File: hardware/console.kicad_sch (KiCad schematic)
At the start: 35 parts, among them J1 USB-C_Module, J2 4.5V_BAT, J3 SWD, J4 UART, Q1 AO3401A, SW1 SW_LEFT, SW2 SW_RIGHT, SW3 SW_UP, SW4 SW_DOWN, SW5 SW_A, SW6 SW_B, U1 STM32G030C8T6, U2 XC6206P332MR

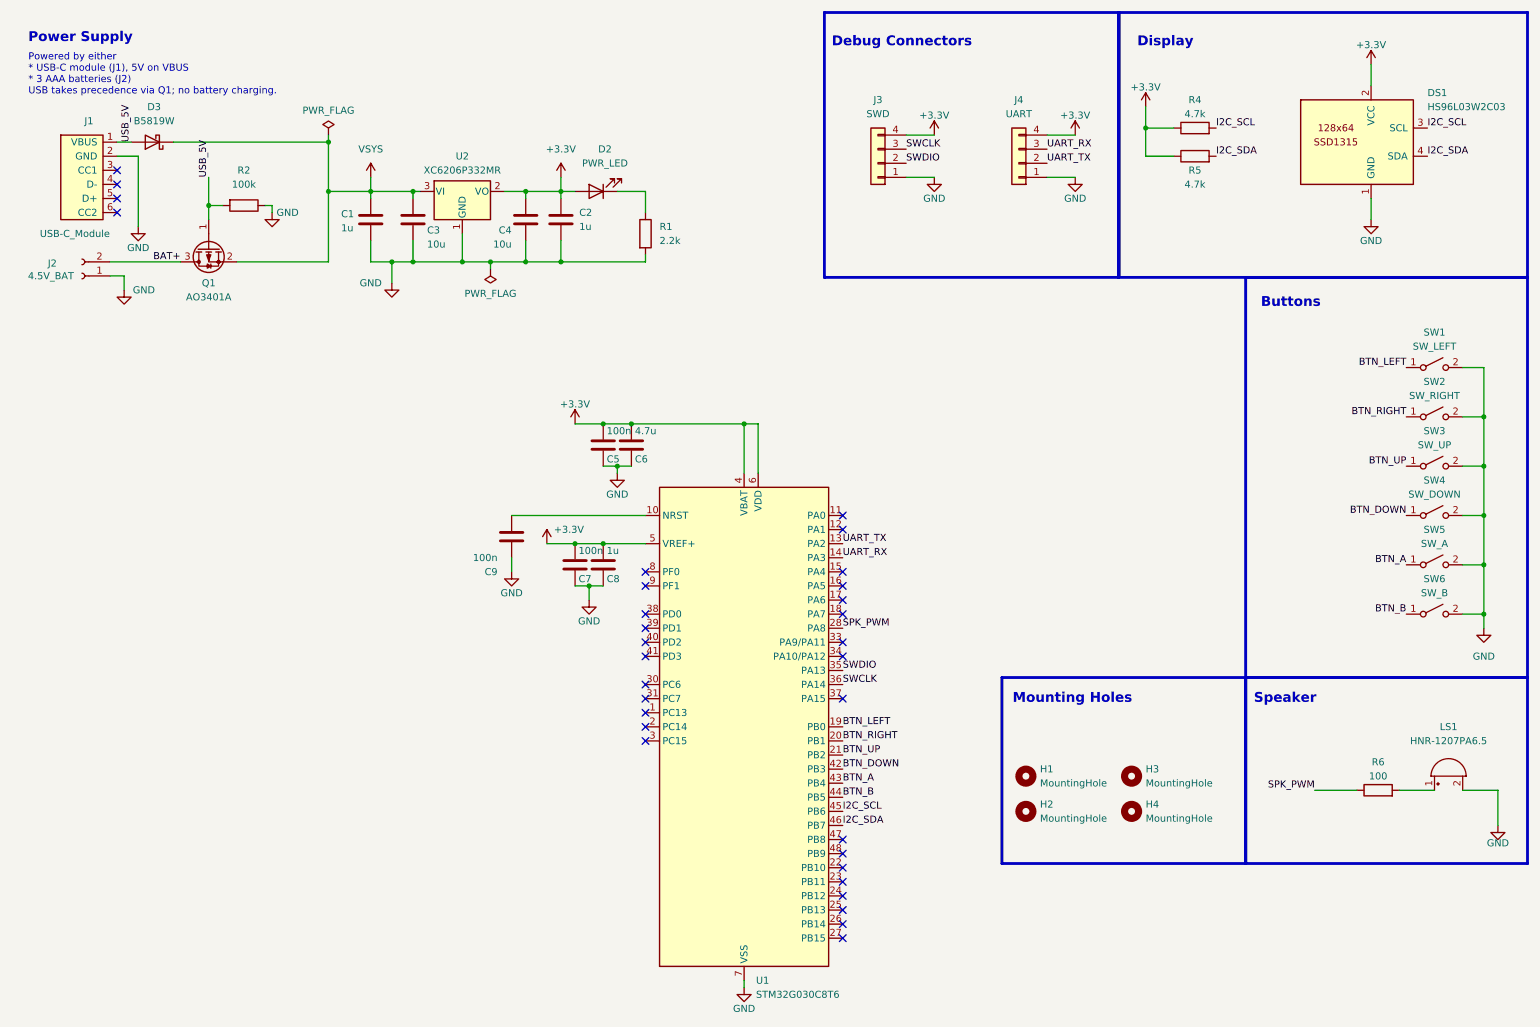
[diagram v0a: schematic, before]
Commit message: checkpoint
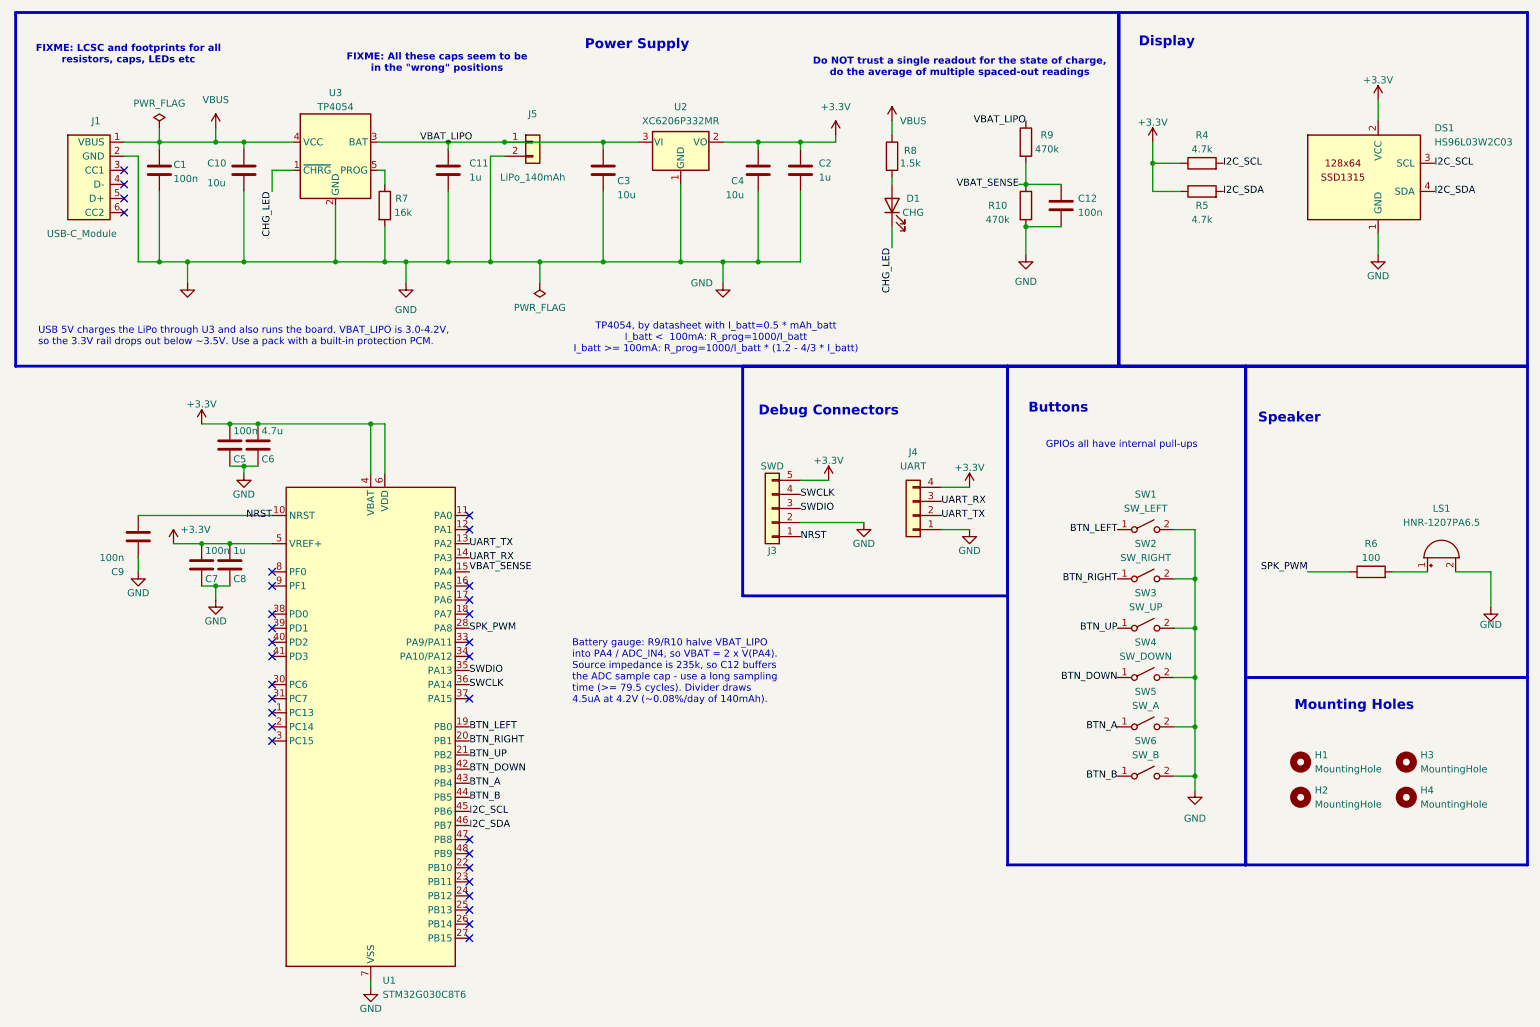
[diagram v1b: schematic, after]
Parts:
- removed D2: PWR_LED, LED_SMD:LED_0603_1608Metric, symbol Device:LED
- removed D3: B5819W, Diode_SMD:D_SOD-123, symbol Device:D_Schottky
- removed J2: 4.5V_BAT, Connector_JST:JST_PH_S2B-PH-K_1x02_P2.00mm_Horizontal, symbol Connector:Conn_01x02_Socket
- removed J3: SWD, Connector_PinHeader_2.54mm:PinHeader_1x04_P2.54mm_Vertical, symbol Connector_Generic:Conn_01x04
- removed Q1: AO3401A, Package_TO_SOT_SMD:SOT-23, symbol Transistor_FET:Q_PMOS_GSD
- removed R1: 2.2k, Resistor_SMD:R_0402_1005Metric, symbol Device:R
- removed R2: 100k, Resistor_SMD:R_0402_1005Metric, symbol Device:R
- added C10: 10u, Capacitor_SMD:C_0805_2012Metric, symbol Device:C
- added C11: 1u, Capacitor_SMD:C_0402_1005Metric, symbol Device:C
- added C12: 100n, Capacitor_SMD:C_0402_1005Metric, symbol Device:C
- added D1: CHG, LED_SMD:LED_0603_1608Metric, symbol Device:LED
- added J3: SWD, Connector_PinHeader_2.54mm:PinHeader_1x05_P2.54mm_Vertical, symbol Connector_Generic:Conn_01x05
- added J5: LiPo_140mAh, Connector_JST:JST_PH_B2B-PH-K_1x02_P2.00mm_Vertical, symbol Connector_Generic:Conn_01x02
- added R10, R9: 470k, Resistor_SMD:R_0402_1005Metric, symbol Device:R
- added R7: 16k, Resistor_SMD:R_0402_1005Metric, symbol Device:R
- added R8: 1.5k, Resistor_SMD:R_0402_1005Metric, symbol Device:R
- added U3: TP4054, Package_TO_SOT_SMD:SOT-23-5, symbol console:TP4054
- C1: value 1u -> 100n
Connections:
- net +3.3V: now also J3.5 (Pin_5)
- net GND: now also C10.2, C11.2, C12.2, J3.2 (Pin_2), J5.2 (Pin_2), R10.2, R7.2, U3.2 (GND)
- net SWCLK: now also J3.4 (Pin_4)
- net SWDIO: now also J3.3 (Pin_3)
- net NRST: now reaches C9.1, U1.10 (NRST)
- net NRST: now also J3.1 (Pin_1)
- net VBAT_SENSE: now reaches U1.15 (PA4)
- net VBAT_SENSE: now also C12.1, R10.1, R9.2
- net USB_5V renamed VBUS
- net VBUS: now also C1.1, C10.1, R8.1, U3.4 (VCC)
- net VSYS renamed VBAT_LIPO
- net VBAT_LIPO: now also C11.1, J5.1 (Pin_1), R9.1, U3.3 (BAT); no longer C1.1
- new net: R7.1, U3.5 (PROG)
- new net: D1.2 (A), R8.2
- new net CHG_LED: D1.1 (K), U3.1 (~{CHRG})
- no-connect marks 32 -> 31
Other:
- note added: "Battery gauge: R9/R10 halve VBAT_LIPO into PA4 / ADC_IN4, so VBAT = 2 x V(PA4). Source impedance is 235k, so C12 buffers the ADC sample cap - use a long sampling time (>= 79.5 cycles). Divider draws 4.5uA at 4.2V (~0.08%/day of 140mAh)."
- note added: "Do NOT trust a single readout for the state of charge, do the average of multiple spaced-out readings"
- note added: "FIXME: All these caps seem to be in the "wrong" positions"
- note added: "FIXME: LCSC and footprints for all resistors, caps, LEDs etc"
- note added: "GPIOs all have internal pull-ups"
- note added: "TP4054, by datasheet with I_batt=0.5 * mAh_batt I_batt < 100mA: R_prog=1000/I_batt I_batt >= 100mA: R_prog=1000/I_batt * (1.2 - 4/3 * I_batt)"
- note added: "USB 5V charges the LiPo through U3 and also runs the board. VBAT_LIPO is 3.0-4.2V, so the 3.3V rail drops out below ~3.5V. Use a pack with a built-in protection PCM."
- note removed: "Powered by either * USB-C module (J1), 5V on VBUS * 3 AAA batteries (J2) USB takes precedence via Q1; no battery charging."
- title: (none) -> MicroConsole
- moved on the sheet: C1, C2, C3, C4, C5, C6, C7, C8, C9, DS1, H1, H2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
